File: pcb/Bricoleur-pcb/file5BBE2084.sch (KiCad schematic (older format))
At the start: 27 parts, among them J2 Conn_02x10_Odd_Even, SW3 SW_Push, SW4 SW_Push, SW5 SW_Push

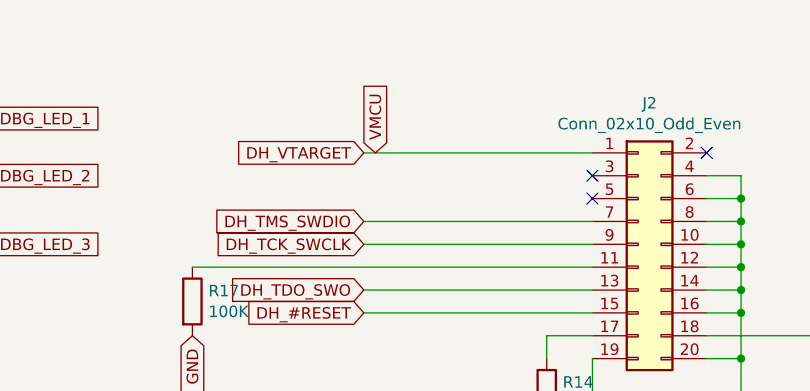
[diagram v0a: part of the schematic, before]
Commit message: PCB…
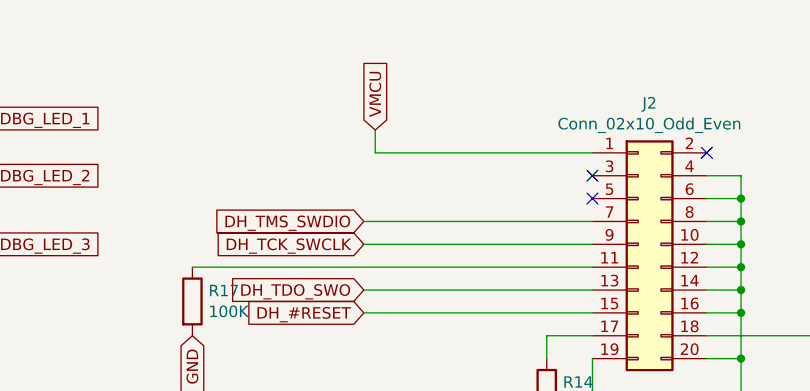
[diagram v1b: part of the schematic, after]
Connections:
- net DH_VTARGET renamed VMCU
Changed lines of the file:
@@
 Text GLabel 8650 2950 3    50   Input ~ 0
 GND
-Text GLabel 7850 1700 0    50   Input ~ 0
-DH_VTARGET
 Text GLabel 7850 2000 0    50   Input ~ 0
 DH_TMS_SWDIO
@@
 Text GLabel 7100 2500 3    50   Input ~ 0
 GND
-Text GLabel 7900 1700 1    50   Input ~ 0
+Text GLabel 7900 1600 1    50   Input ~ 0
 VMCU
 NoConn ~ 9350 1700
@@
 	7850 2100 8850 2100
 Wire Wire Line
-	7850 1700 8850 1700
-Wire Wire Line
 	7850 2000 8850 2000
 Text GLabel 8400 4750 0    50   Input ~ 0
@@
 	7350 5200 7350 5000
 Connection ~ 8600 5200
+Wire Wire Line
+	7900 1700 7900 1600
+Wire Wire Line
+	7900 1700 8850 1700
 $EndSCHEMATC

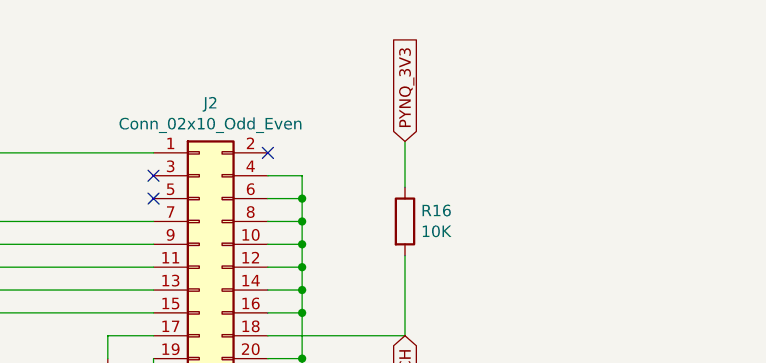
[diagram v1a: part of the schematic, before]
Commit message: Overwrite
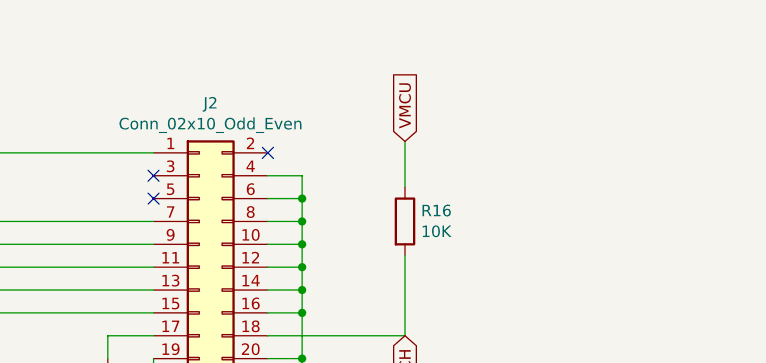
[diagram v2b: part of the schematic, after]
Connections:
- net PYNQ_3V3 is gone; now on net VMCU: R16.1
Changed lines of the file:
@@
 GND
 Text GLabel 9950 1650 1    50   Input ~ 0
-PYNQ_3V3
+VMCU
 $Comp
 L Device:R R16
